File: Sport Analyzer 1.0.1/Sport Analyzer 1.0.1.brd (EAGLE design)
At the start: 122.7 x 68.6 mm, 26 parts, among them IC2 7805DT, Q1 MMBT4403, U1 HX711

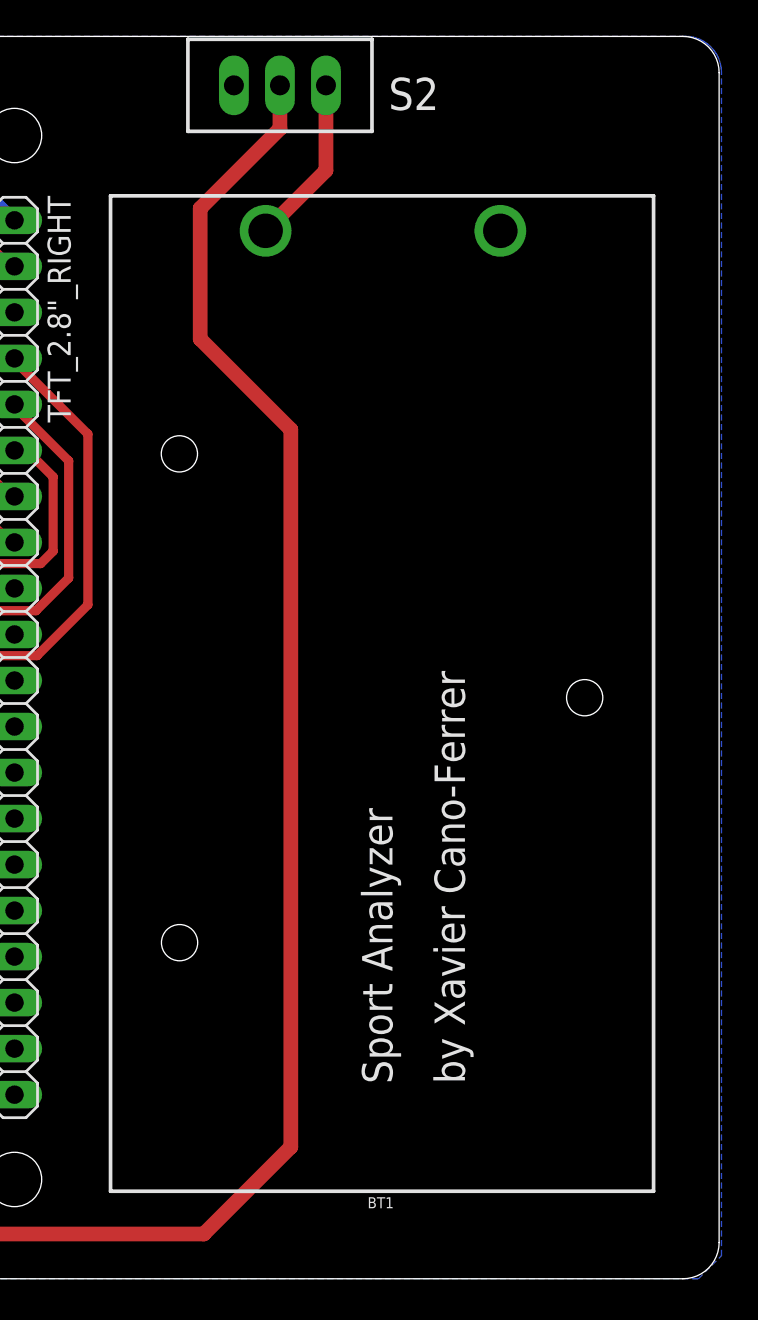
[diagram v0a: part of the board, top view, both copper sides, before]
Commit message: SA 1.0.1 (4)
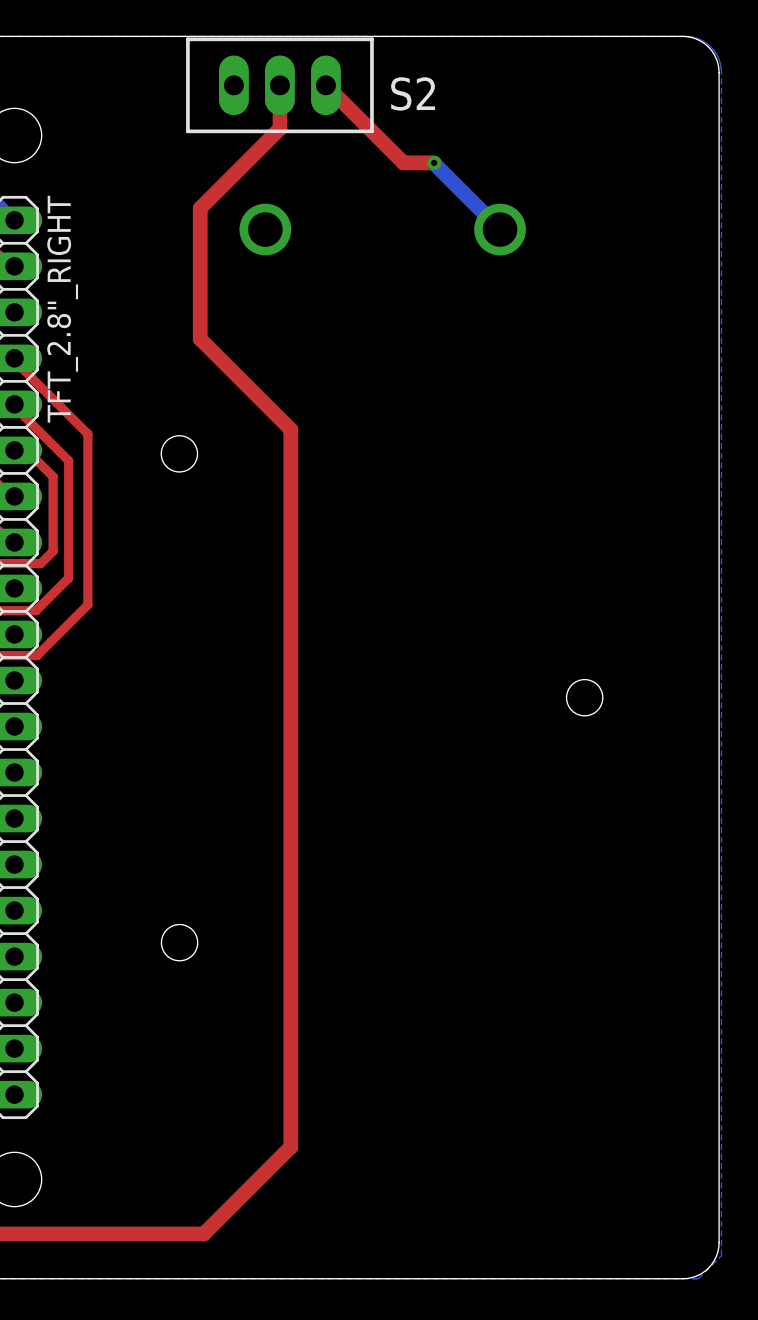
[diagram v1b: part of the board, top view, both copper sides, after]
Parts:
- moved BT1 12.9 mm to (109.3, 56.6), flipped to the bottom
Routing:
- net N$42: track 9.41 -> 12.9 mm, vias 0 -> 1
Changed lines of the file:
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@@
 <hole x="82.55" y="61.83" drill="3"/>
 <hole x="6.25" y="4.21" drill="3"/>
-<text x="103.41" y="9.49" size="1.6764" layer="25" rot="R90">Sport Analyzer</text>
+<text x="104.88" y="20.51" size="1.6764" layer="26" rot="MR90">Sport Analyzer</text>
 <hole x="91.65" y="44.26" drill="2"/>
 <hole x="114.02" y="30.8" drill="2"/>
 <hole x="91.66" y="17.28" drill="2"/>
-<text x="107.41" y="9.49" size="1.6764" layer="25" rot="R90">by Xavier Cano-Ferrer</text>
+<text x="101.18" y="20.51" size="1.6764" layer="26" rot="MR90">by Xavier Cano-Ferrer</text>
 </plain>
 <attributes>
@@
 <attribute name="VALUE" x="43.352" y="57.32" size="1.27" layer="27" ratio="10"/>
 </element>
-<element name="BT1" library="SparkFun-Batteries" package="BATTCON_9V" value="" x="96.41" y="56.57" smashed="yes" rot="R90">
-<attribute name="NAME" x="102.76" y="3.23" size="0.6096" layer="25" font="vector" ratio="20" rot="R180" align="bottom-center"/>
-<attribute name="PROD_ID" value="BATT-10855" x="96.41" y="56.57" size="1.778" layer="27" rot="R90" display="off"/>
-<attribute name="VALUE" x="102.76" y="31.17" size="0.6096" layer="27" font="vector" ratio="20" rot="R180" align="top-center"/>
+<element name="BT1" library="SparkFun-Batteries" package="BATTCON_9V" value="" x="109.35" y="56.64" smashed="yes" rot="MR90">
+<attribute name="NAME" x="103" y="3.3" size="0.6096" layer="26" font="vector" ratio="20" rot="MR180" align="bottom-center"/>
+<attribute name="PROD_ID" value="BATT-10855" x="109.35" y="56.64" size="1.778" layer="28" rot="MR90" display="off"/>
+<attribute name="VALUE" x="103" y="31.24" size="0.6096" layer="28" font="vector" ratio="20" rot="MR180" align="top-center"/>
 </element>
 <element name="S2" library="switch" library_urn="urn:adsk.eagle:library:380" package="TL3XPO" package3d_urn="urn:adsk.eagle:package:27745/1" value="TL32PO" x="97.2" y="64.6" smashed="yes" rot="R180">
@@
 <contactref element="S2" pad="1"/>
 <contactref element="BT1" pad="+"/>
-<wire x1="96.41" y1="56.57" x2="99.74" y2="59.9" width="0.8128" layer="1"/>
-<wire x1="99.74" y1="59.9" x2="99.74" y2="64.6" width="0.8128" layer="1"/>
+<wire x1="109.35" y1="56.64" x2="105.71" y2="60.28" width="0.8128" layer="16"/>
+<wire x1="105.71" y1="60.28" x2="105.71" y2="60.32" width="0.8128" layer="16"/>
+<wire x1="105.71" y1="60.32" x2="104.02" y2="60.32" width="0.8128" layer="1"/>
+<wire x1="104.02" y1="60.32" x2="99.74" y2="64.6" width="0.8128" layer="1"/>
+<via x="105.71" y="60.32" extent="1-16" drill="0.35"/>
 </signal>
 <signal name="N$9">
